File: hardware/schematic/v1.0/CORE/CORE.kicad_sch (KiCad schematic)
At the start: 77 parts, among them J1 Conn_01x03_Socket, J10 USB_C_Receptacle_USB2.0_16P, J11 Conn_01x06_Socket, J2 Conn_Coaxial, J3 Conn_Coaxial, J4 Conn_Coaxial, J5 Conn_Coaxial, J6 Conn_Coaxial, J7 Conn_Coaxial, J8 Conn_Coaxial, J9 Conn_Coaxial, M1 ZYNQ7010&7020, U1 TXS02612RTWR, U2 SP3232, U3 SD_Card, U4 AMS1117-2.5, U5 AMS1117-1.8

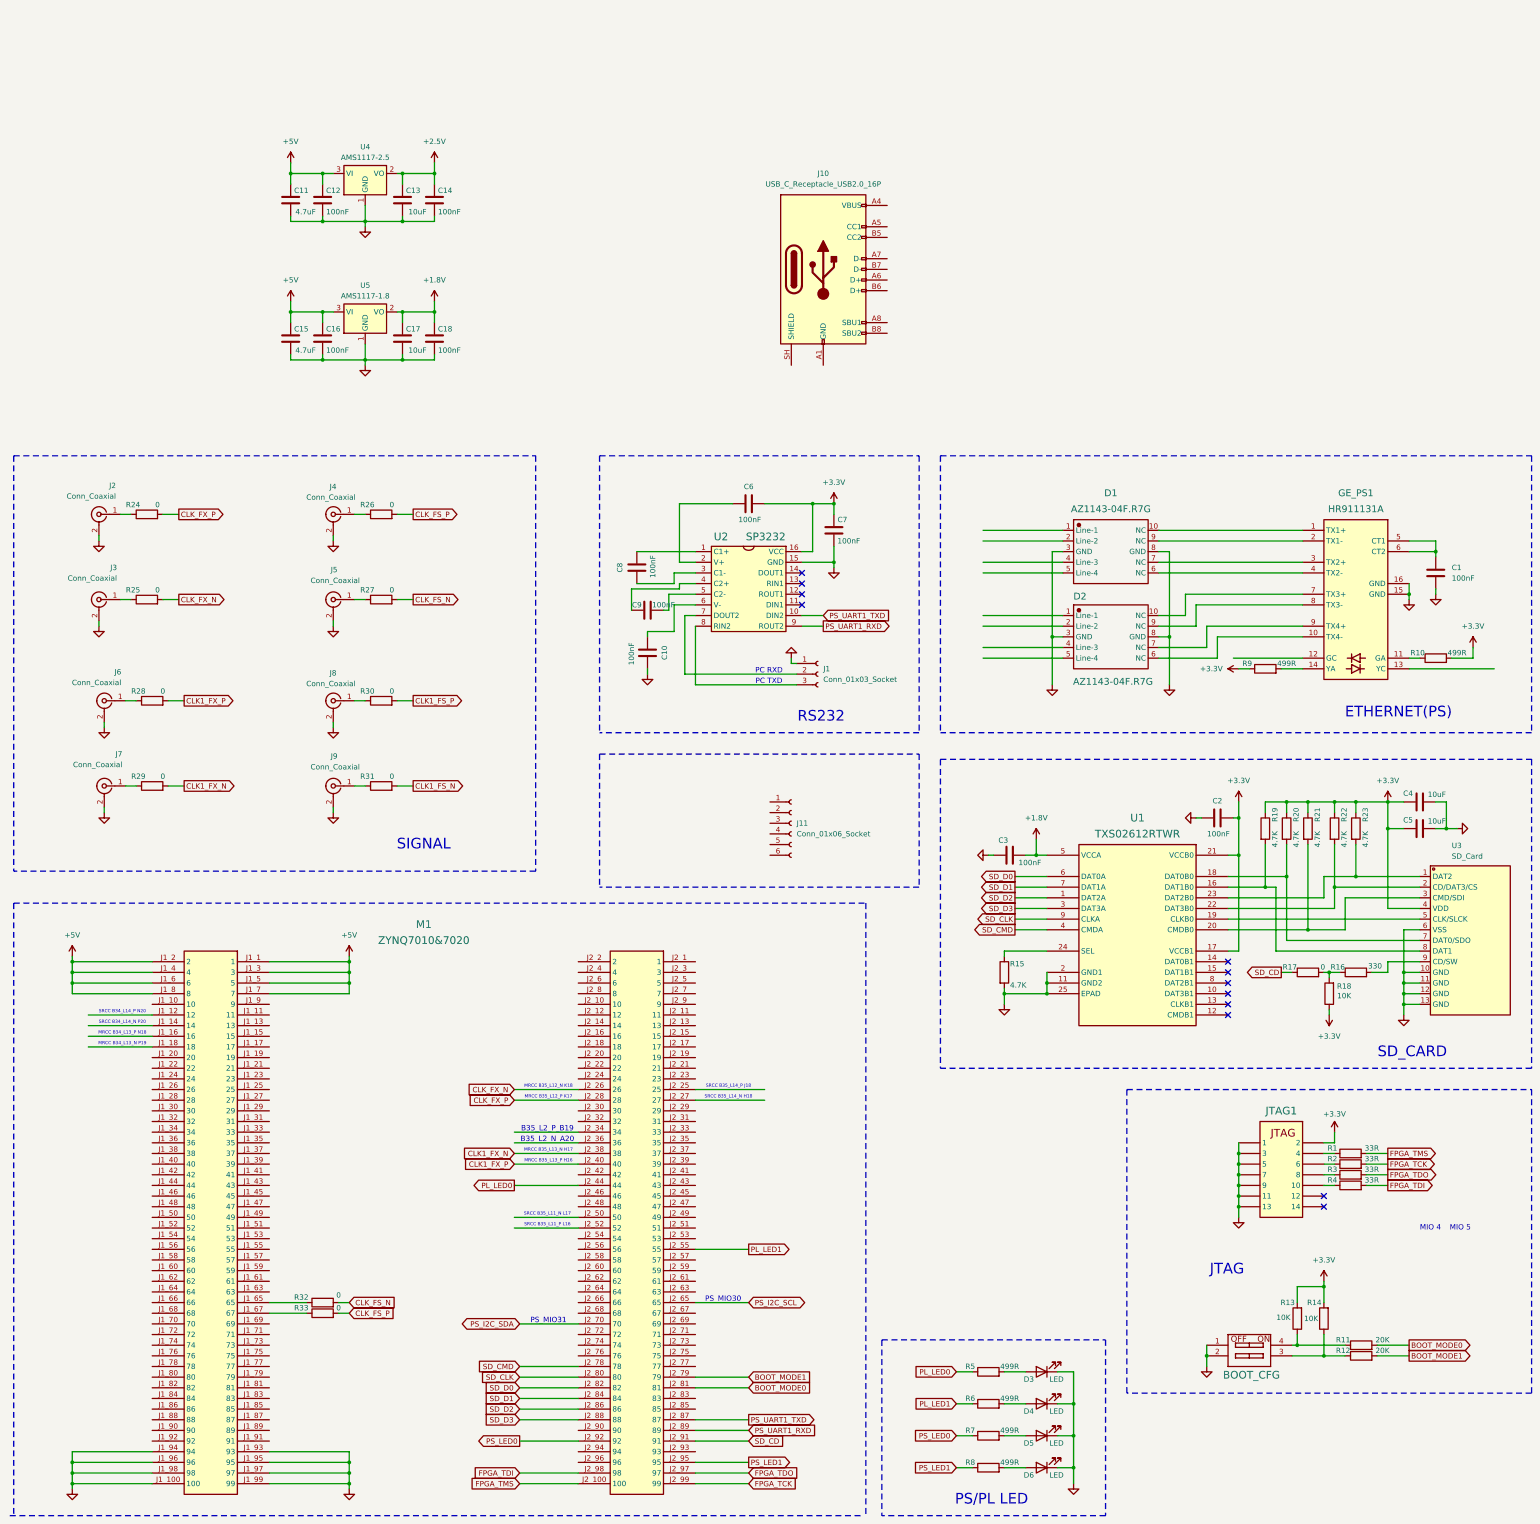
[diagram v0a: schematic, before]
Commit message: sch update
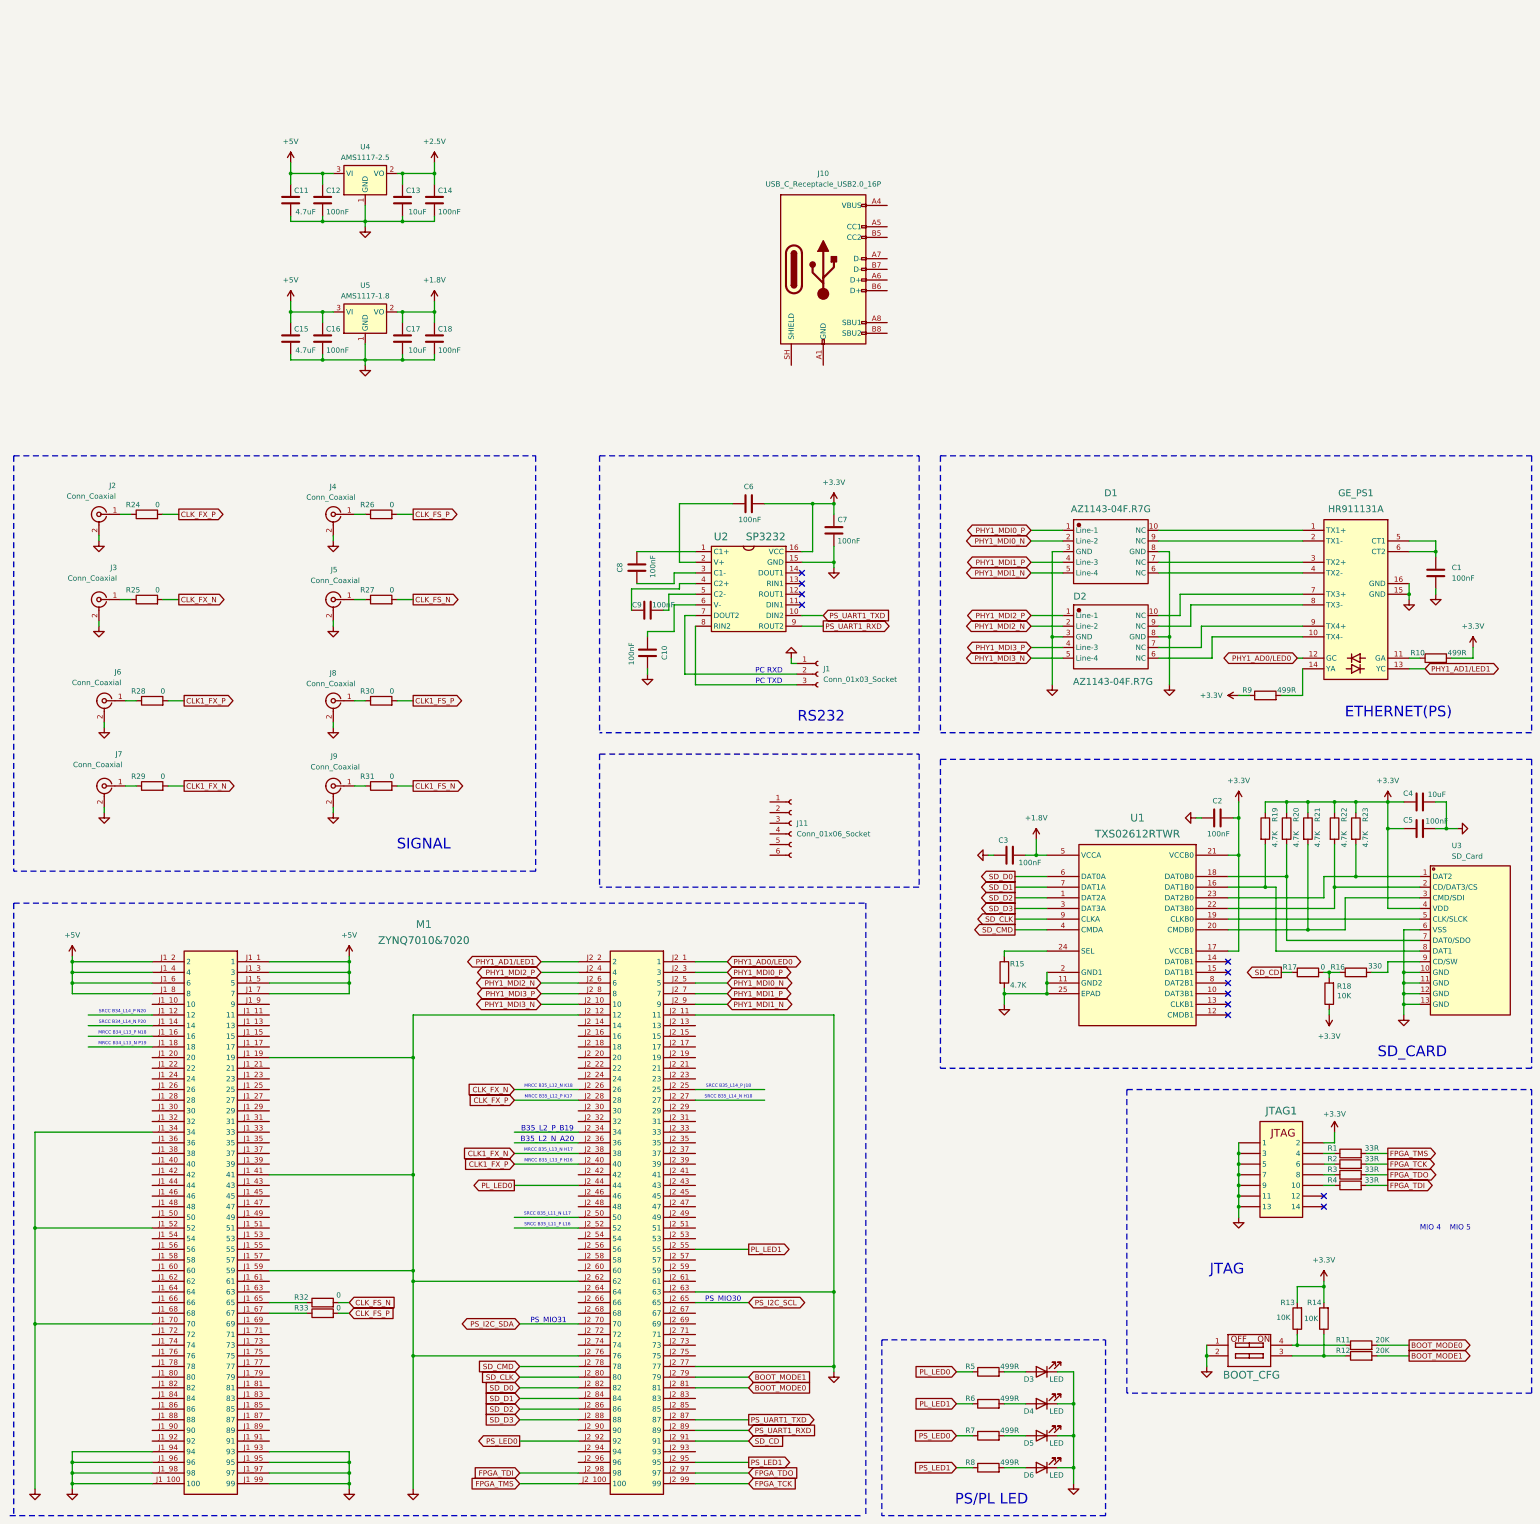
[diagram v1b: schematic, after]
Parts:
- C5: value 10uF -> 100nF
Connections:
- net GND: now also M1.J1_19 (19), M1.J1_34 (34), M1.J1_41 (41), M1.J1_52 (52), M1.J1_59 (59), M1.J1_70 (70), M1.J2_11 (11), M1.J2_12 (12), M1.J2_62 (62), M1.J2_63 (63), M1.J2_76 (76), M1.J2_77 (77)
- net PHY1_AD0/LED0: now reaches M1.J2_1 (1)
- net PHY1_AD0/LED0: now also GE_PS1.12 (GC)
- net PHY1_MDI3_N: now reaches M1.J2_10 (10)
- net PHY1_MDI3_N: now also D2.5 (Line-4)
- net PHY1_AD1/LED1: now reaches M1.J2_2 (2)
- net PHY1_AD1/LED1: now also GE_PS1.13 (YC)
- net PHY1_MDI0_P: now reaches M1.J2_3 (3)
- net PHY1_MDI0_P: now also D1.1 (Line-1)
- net PHY1_MDI2_P: now reaches M1.J2_4 (4)
- net PHY1_MDI2_P: now also D2.1 (Line-1)
- net PHY1_MDI0_N: now reaches M1.J2_5 (5)
- net PHY1_MDI0_N: now also D1.2 (Line-2)
- net PHY1_MDI2_N: now reaches M1.J2_6 (6)
- net PHY1_MDI2_N: now also D2.2 (Line-2)
- net PHY1_MDI1_P: now reaches M1.J2_7 (7)
- net PHY1_MDI1_P: now also D1.4 (Line-3)
- net PHY1_MDI3_P: now reaches M1.J2_8 (8)
- net PHY1_MDI3_P: now also D2.4 (Line-3)
- net PHY1_MDI1_N: now reaches M1.J2_9 (9)
- net PHY1_MDI1_N: now also D1.5 (Line-4)
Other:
- moved on the sheet: R9

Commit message: sch update
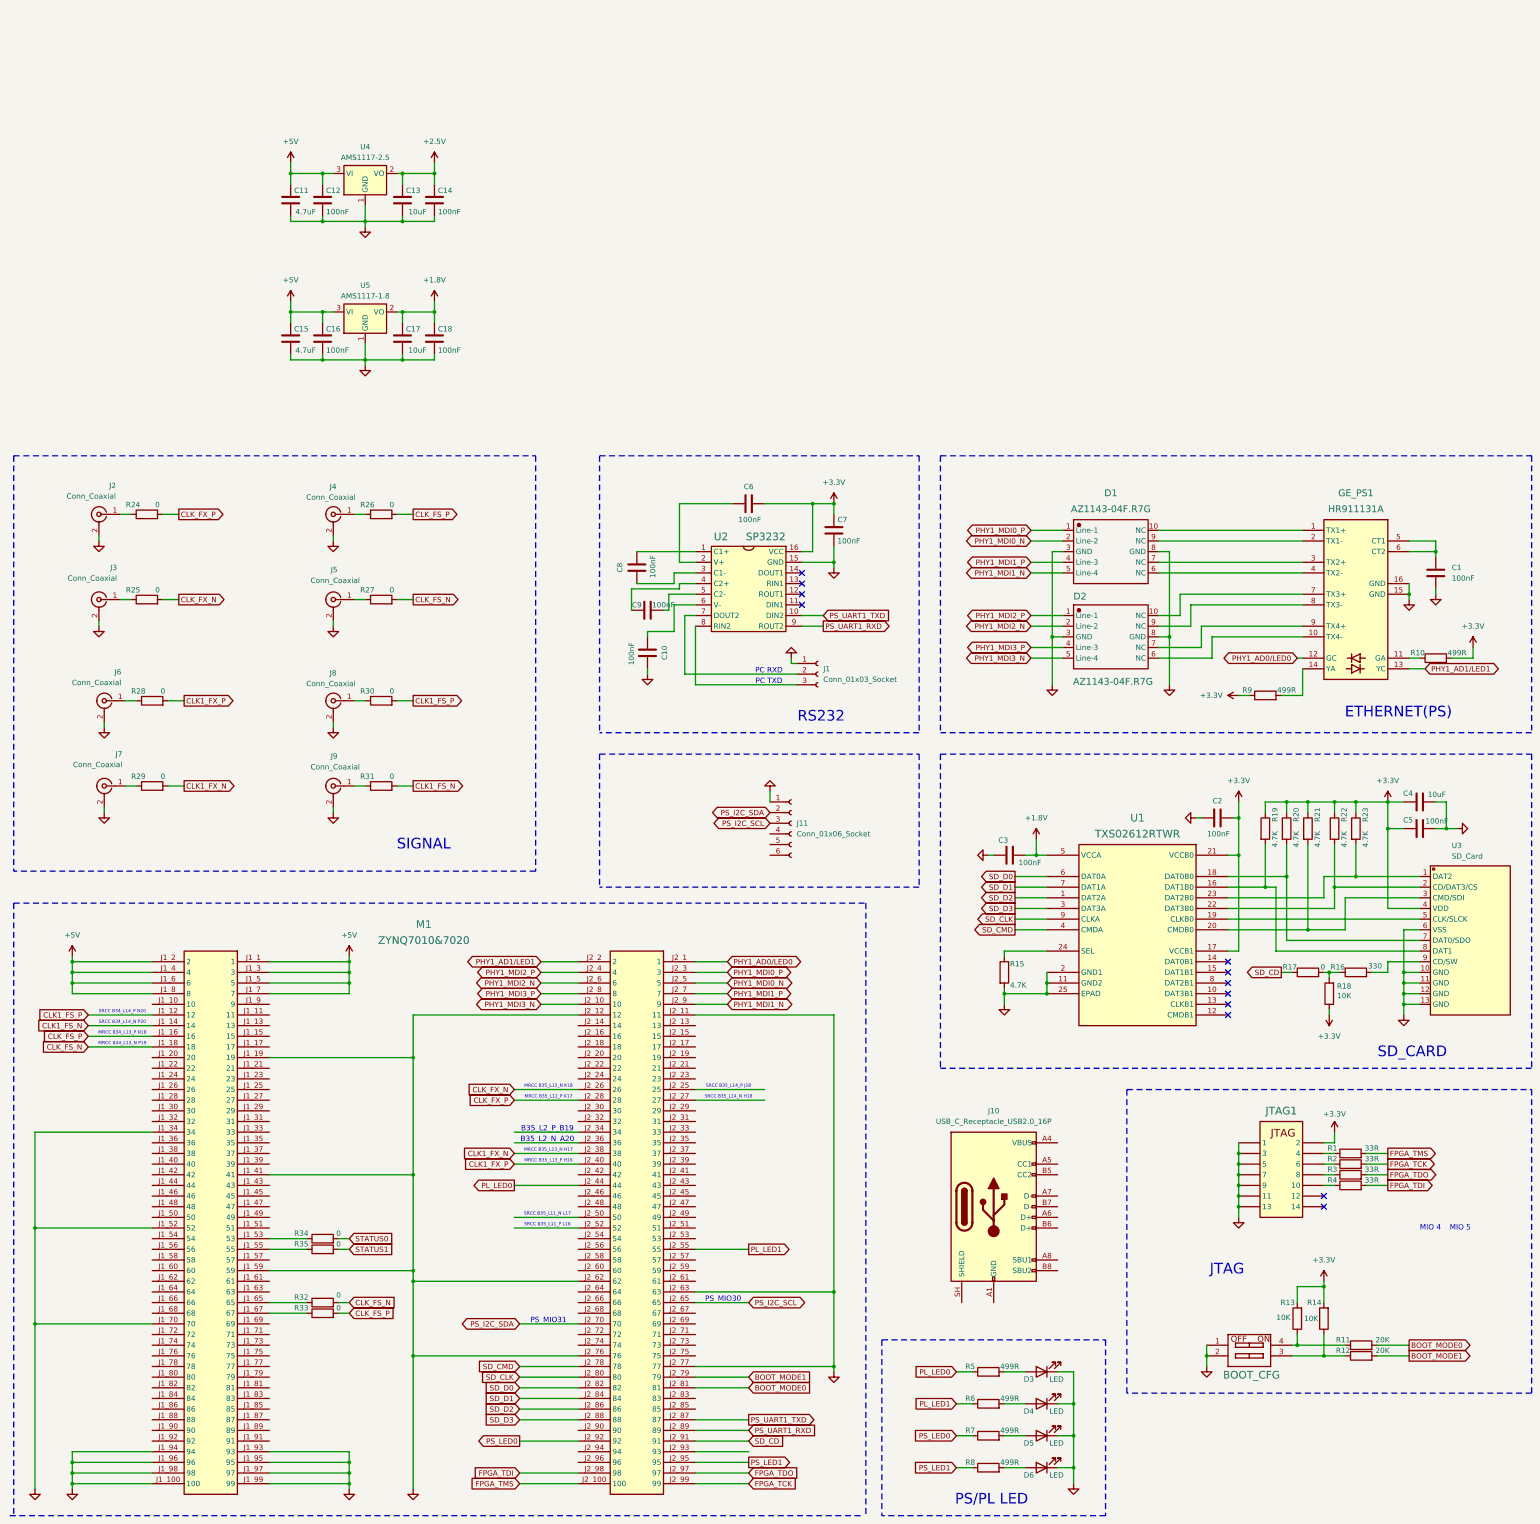
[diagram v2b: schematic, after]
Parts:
- added R34, R35: 0, Resistor_SMD:R_0402_1005Metric, symbol Device:R
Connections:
- net CLK1_FS_N: now also M1.J1_14 (14)
- net CLK1_FS_P: now also M1.J1_12 (12)
- net CLK_FS_N: now also M1.J1_18 (18)
- net CLK_FS_P: now also M1.J1_16 (16)
- net GND: now also J11.1 (Pin_1)
- net PS_I2C_SCL: now also J11.3 (Pin_3)
- net PS_I2C_SDA: now also J11.2 (Pin_2)
- net at M1.J1_53 (53): now also R34.1
- net at M1.J1_55 (55): now also R35.1
- new net STATUS0: R34.2
- new net STATUS1: R35.2
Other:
- moved on the sheet: J10
